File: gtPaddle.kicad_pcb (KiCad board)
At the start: 2 copper layers, 139.7 x 57.2 mm, 50 parts, among them IC1 74157N, IC2 74157N, J1 Conn_01x02_Pin, J2 Conn_01x02_Pin, J3 Conn_01x02_Pin, J4 Conn_01x02_Pin, Q1 2N3904, Q10 2N3904, Q2 2N3904, Q3 2N3904, Q9 2N3904, U1 ADC0804LCN

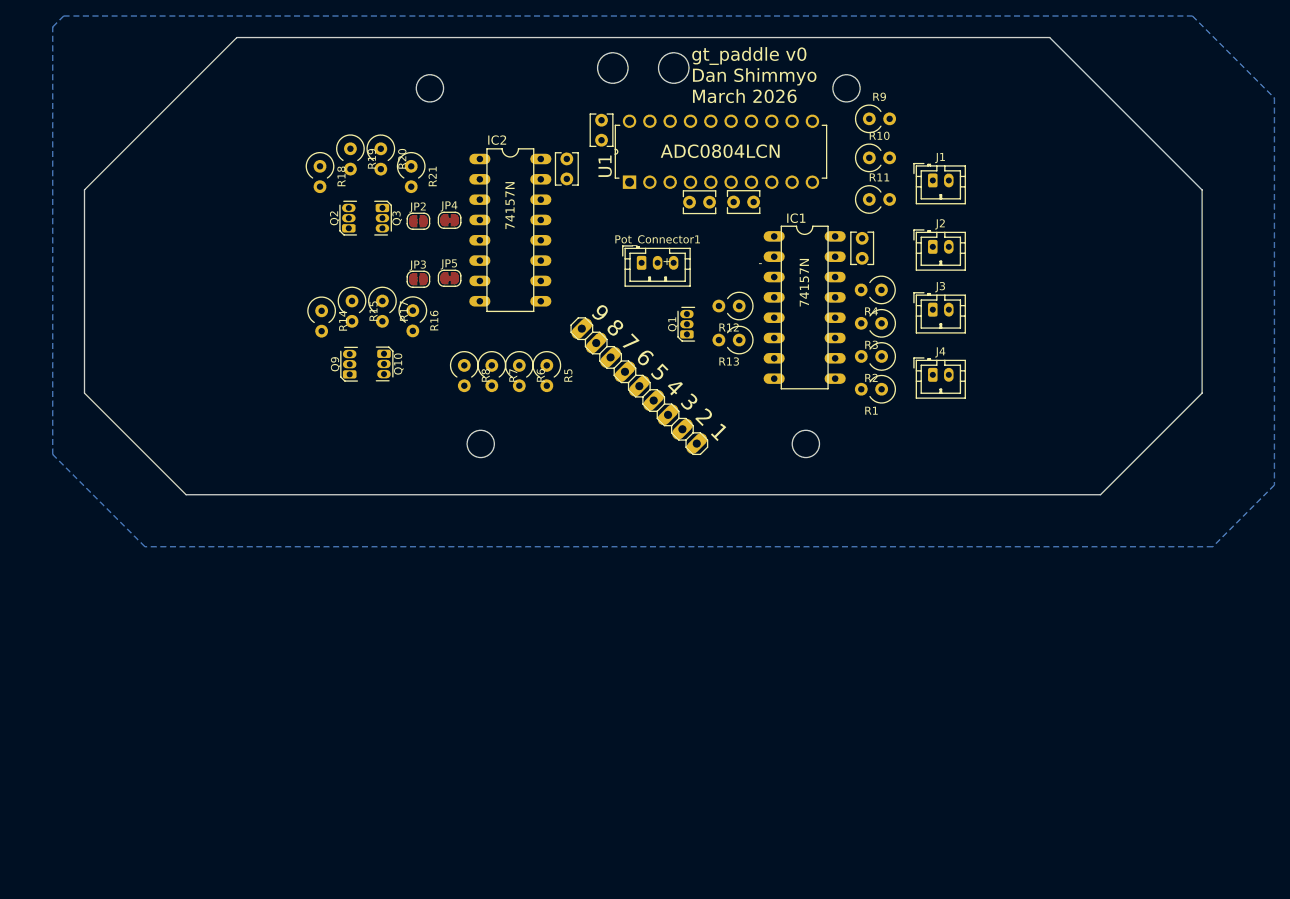
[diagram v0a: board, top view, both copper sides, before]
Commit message: compact layout
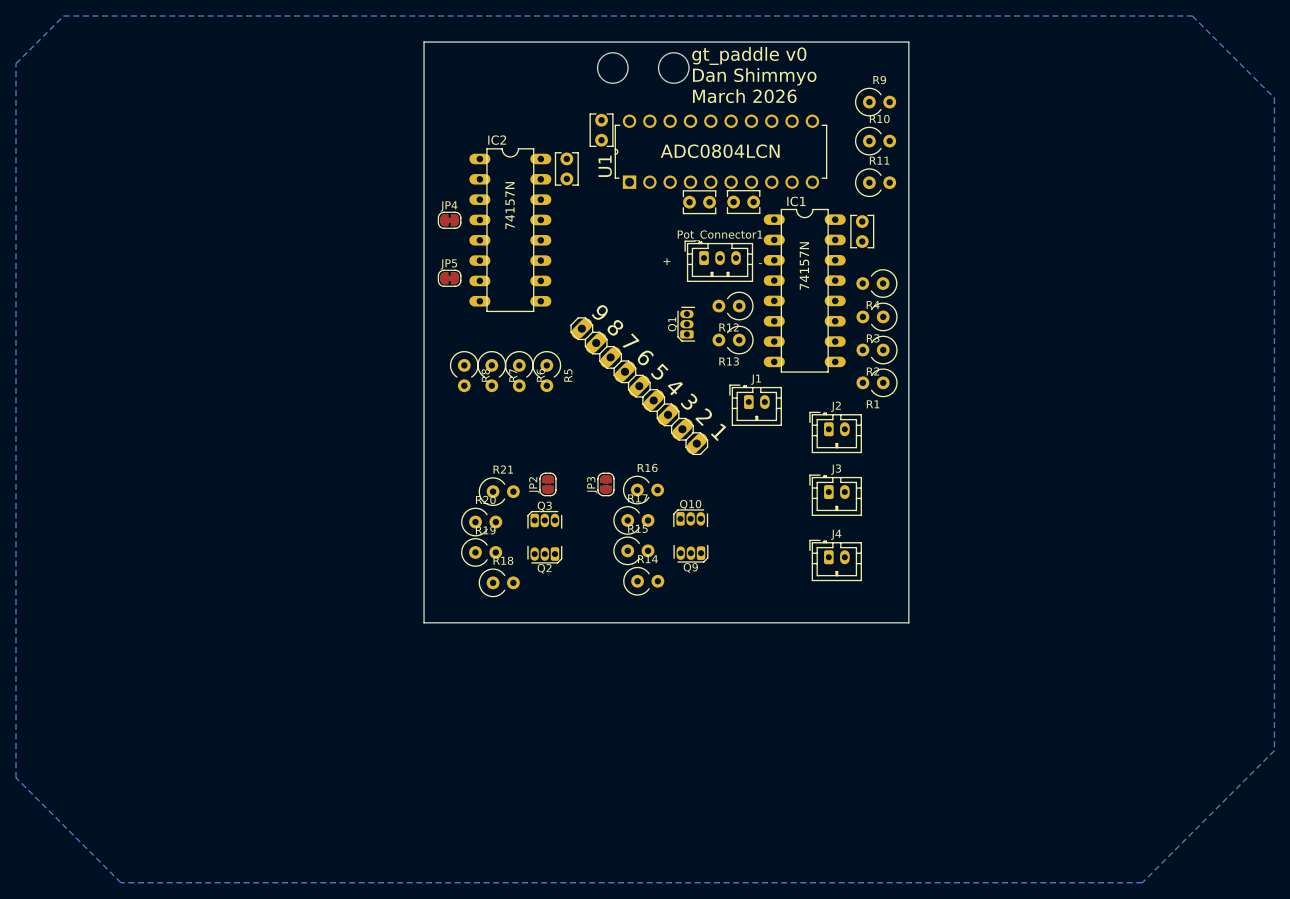
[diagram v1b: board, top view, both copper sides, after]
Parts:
- removed @HOLE0, @HOLE1, @HOLE2, @HOLE3: , 
- moved R18 56.4 mm to (124.8, 135.2), turned to 0 degrees
- moved R19 52.8 mm to (122.6, 131.4), turned to 0 degrees
- moved R14 52.0 mm to (142.9, 135.0), turned to 0 degrees
- moved Q9 49.3 mm to (150.8, 131.5), turned to 180 degrees
- moved Q2 48.2 mm to (132.6, 131.6), turned to 180 degrees
- moved R20 48.1 mm to (122.6, 127.6), turned to 0 degrees
- moved R15 46.5 mm to (141.7, 131.2), turned to 0 degrees
- moved Q3 43.5 mm to (130.0, 127.4), turned to 0 degrees
- moved Q10 42.4 mm to (148.3, 127.2), turned to 0 degrees
- moved R21 41.9 mm to (124.8, 123.8), turned to 0 degrees
- moved R17 41.1 mm to (141.7, 127.4), turned to 0 degrees
- moved JP2 36.7 mm to (131.7, 122.9), turned to 90 degrees
- moved J1 36.0 mm to (156.8, 112.6)
- moved R16 35.9 mm to (142.9, 123.6), turned to 0 degrees
- moved JP3 34.7 mm to (138.9, 122.9), turned to 90 degrees
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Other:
- board size 139.7 x 57.2 mm -> 60.6 x 72.6 mm
